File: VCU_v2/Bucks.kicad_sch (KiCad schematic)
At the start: 16 parts, among them U1 TPS5430

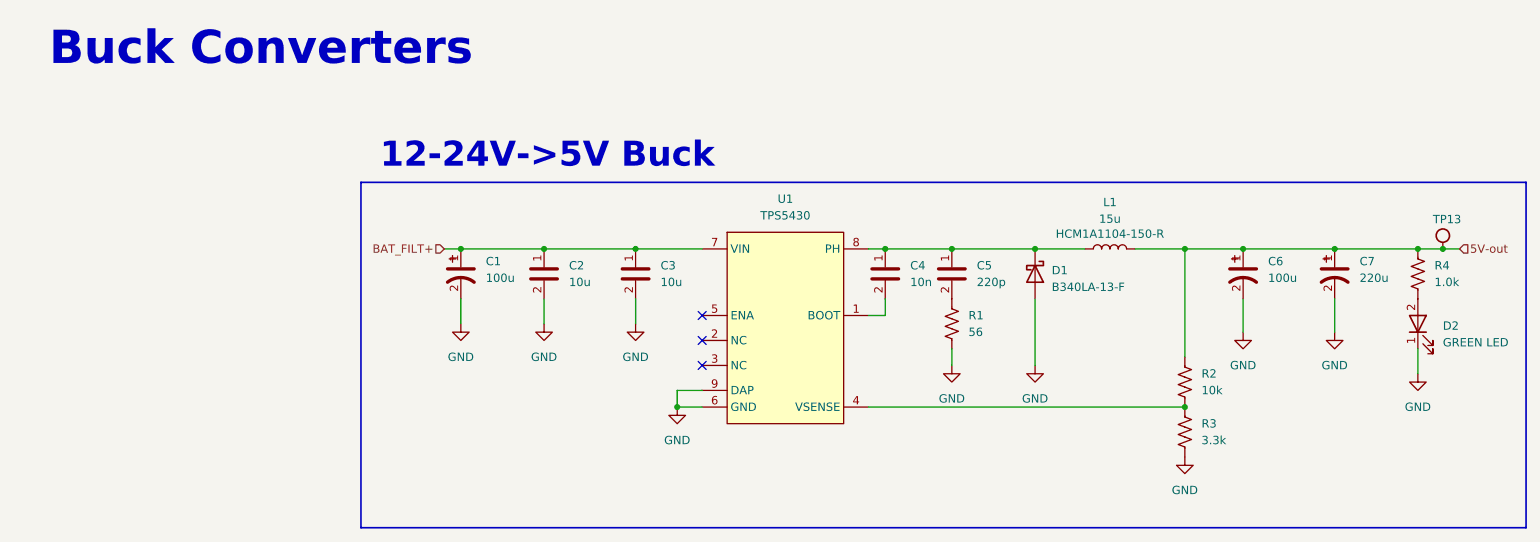
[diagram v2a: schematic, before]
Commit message: placements friggin 80% friggin done shoutout epstein
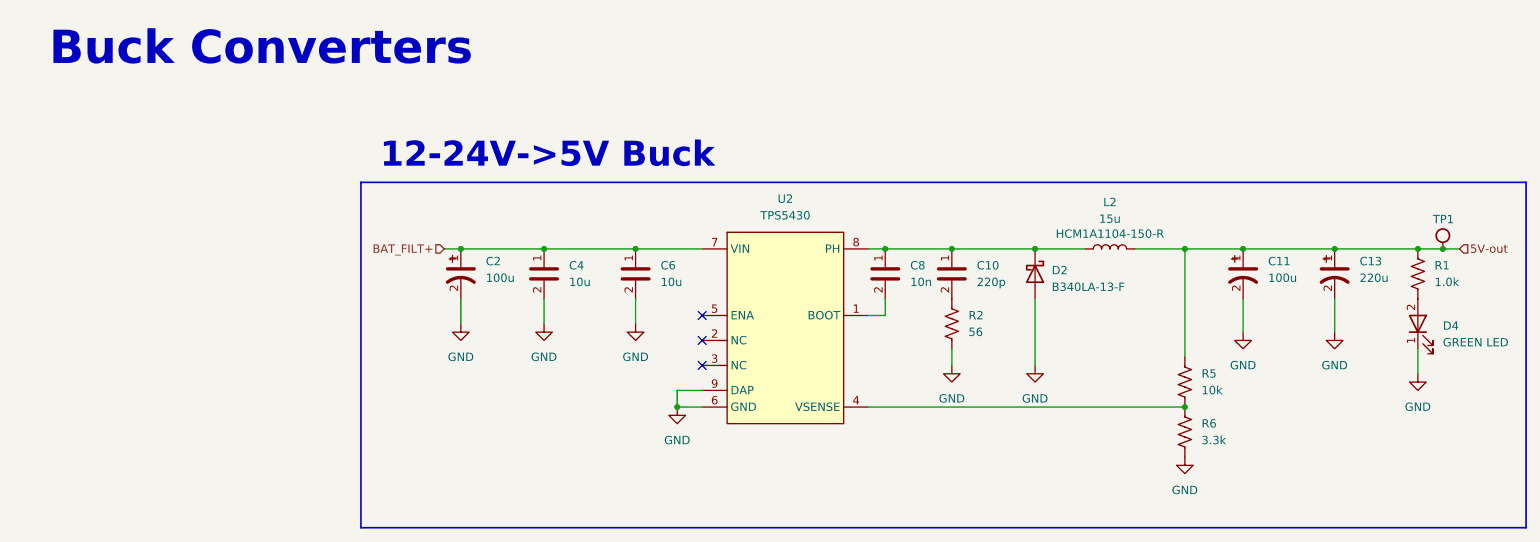
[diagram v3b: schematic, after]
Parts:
- renumbered C5 to C10, C6 to C11, C7 to C13, C1 to C2, C2 to C4, C3 to C6, C4 to C8, D1 to D2, D2 to D4, L1 to L2, R4 to R1, R1 to R2, R2 to R5, R3 to R6, TP13 to TP1, U1 to U2
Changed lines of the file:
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@@
 		(dnp no)
 		(fields_autoplaced yes)
-		(property "Reference" "#PWR017"
+		(property "Reference" "#PWR023"
 			(at 186.69 86.36 0)
 			(effects
@@
 			(project ""
 				(path "/4ee6c2ad-9a1b-4276-b3cf-1cc8dc52967e/9e4b5f8d-93dc-46d5-aa92-d0e0d2e07b3d/83ba1e49-760f-4968-9bbd-ff2e6c9ab433"
-					(reference "#PWR017")
+					(reference "#PWR023")
 					(unit 1)
 				)
@@
 		(dnp no)
 		(fields_autoplaced yes)
-		(property "Reference" "#PWR016"
+		(property "Reference" "#PWR021"
 			(at 163.83 72.39 0)
 			(effects
@@
 			(project "VCU_v1"
 				(path "/4ee6c2ad-9a1b-4276-b3cf-1cc8dc52967e/9e4b5f8d-93dc-46d5-aa92-d0e0d2e07b3d/83ba1e49-760f-4968-9bbd-ff2e6c9ab433"
-					(reference "#PWR016")
+					(reference "#PWR021")
 					(unit 1)
 				)
@@
 		(dnp no)
 		(fields_autoplaced yes)
-		(property "Reference" "#PWR012"
+		(property "Reference" "#PWR013"
 			(at 88.9 66.04 0)
 			(effects
@@
 			(project "VCU_v1"
 				(path "/4ee6c2ad-9a1b-4276-b3cf-1cc8dc52967e/9e4b5f8d-93dc-46d5-aa92-d0e0d2e07b3d/83ba1e49-760f-4968-9bbd-ff2e6c9ab433"
-					(reference "#PWR012")
+					(reference "#PWR013")
 					(unit 1)
 				)
@@
 		(dnp no)
 		(fields_autoplaced yes)
-		(property "Reference" "C3"
+		(property "Reference" "C6"
 			(at 106.68 50.7999 0)
 			(effects
@@
 			(project "VCU_v1"
 				(path "/4ee6c2ad-9a1b-4276-b3cf-1cc8dc52967e/9e4b5f8d-93dc-46d5-aa92-d0e0d2e07b3d/83ba1e49-760f-4968-9bbd-ff2e6c9ab433"
-					(reference "C3")
+					(reference "C6")
 					(unit 1)
 				)
@@
 		(on_board yes)
 		(dnp no)
-		(property "Reference" "D1"
+		(property "Reference" "D2"
 			(at 166.37 50.8 90)
 			(effects
@@
 			(project "VCU_v1"
 				(path "/4ee6c2ad-9a1b-4276-b3cf-1cc8dc52967e/9e4b5f8d-93dc-46d5-aa92-d0e0d2e07b3d/83ba1e49-760f-4968-9bbd-ff2e6c9ab433"
-					(reference "D1")
+					(reference "D2")
 					(unit 1)
 				)
@@
 		(dnp no)
 		(fields_autoplaced yes)
-		(property "Reference" "R1"
+		(property "Reference" "R2"
 			(at 153.67 58.4199 90)
 			(effects
@@
 			(project ""
 				(path "/4ee6c2ad-9a1b-4276-b3cf-1cc8dc52967e/9e4b5f8d-93dc-46d5-aa92-d0e0d2e07b3d/83ba1e49-760f-4968-9bbd-ff2e6c9ab433"
-					(reference "R1")
+					(reference "R2")
 					(unit 1)
 				)
@@
 		(dnp no)
 		(fields_autoplaced yes)
-		(property "Reference" "U1"
+		(property "Reference" "U2"
 			(at 125.73 40.64 0)
 			(effects
@@
 			(project "VCU_v1"
 				(path "/4ee6c2ad-9a1b-4276-b3cf-1cc8dc52967e/9e4b5f8d-93dc-46d5-aa92-d0e0d2e07b3d/83ba1e49-760f-4968-9bbd-ff2e6c9ab433"
-					(reference "U1")
+					(reference "U2")
 					(unit 1)
 				)
@@
 		(dnp no)
 		(fields_autoplaced yes)
-		(property "Reference" "C4"
+		(property "Reference" "C8"
 			(at 144.78 50.7999 0)
 			(effects
@@
 			(project "VCU_v1"
 				(path "/4ee6c2ad-9a1b-4276-b3cf-1cc8dc52967e/9e4b5f8d-93dc-46d5-aa92-d0e0d2e07b3d/83ba1e49-760f-4968-9bbd-ff2e6c9ab433"
-					(reference "C4")
+					(reference "C8")
 					(unit 1)
 				)
@@
 		(dnp no)
 		(fields_autoplaced yes)
-		(property "Reference" "#PWR014"
+		(property "Reference" "#PWR017"
 			(at 109.22 78.74 0)
 			(effects
@@
 			(project "VCU_v1"
 				(path "/4ee6c2ad-9a1b-4276-b3cf-1cc8dc52967e/9e4b5f8d-93dc-46d5-aa92-d0e0d2e07b3d/83ba1e49-760f-4968-9bbd-ff2e6c9ab433"
-					(reference "#PWR014")
+					(reference "#PWR017")
 					(unit 1)
 				)
@@
 		(dnp no)
 		(fields_autoplaced yes)
-		(property "Reference" "#PWR015"
+		(property "Reference" "#PWR019"
 			(at 151.13 72.39 0)
 			(effects
@@
 			(project "VCU_v1"
 				(path "/4ee6c2ad-9a1b-4276-b3cf-1cc8dc52967e/9e4b5f8d-93dc-46d5-aa92-d0e0d2e07b3d/83ba1e49-760f-4968-9bbd-ff2e6c9ab433"
-					(reference "#PWR015")
+					(reference "#PWR019")
 					(unit 1)
 				)
@@
 		(on_board yes)
 		(dnp no)
-		(property "Reference" "L1"
+		(property "Reference" "L2"
 			(at 175.26 41.148 90)
 			(effects
@@
 			(project ""
 				(path "/4ee6c2ad-9a1b-4276-b3cf-1cc8dc52967e/9e4b5f8d-93dc-46d5-aa92-d0e0d2e07b3d/83ba1e49-760f-4968-9bbd-ff2e6c9ab433"
-					(reference "L1")
+					(reference "L2")
 					(unit 1)
 				)
@@
 		(dnp no)
 		(fields_autoplaced yes)
-		(property "Reference" "R3"
+		(property "Reference" "R6"
 			(at 189.23 74.9299 90)
 			(effects
@@
 			(project ""
 				(path "/4ee6c2ad-9a1b-4276-b3cf-1cc8dc52967e/9e4b5f8d-93dc-46d5-aa92-d0e0d2e07b3d/83ba1e49-760f-4968-9bbd-ff2e6c9ab433"
-					(reference "R3")
+					(reference "R6")
 					(unit 1)
 				)
@@
 		(dnp no)
 		(fields_autoplaced yes)
-		(property "Reference" "C1"
+		(property "Reference" "C2"
 			(at 80.01 50.1649 0)
 			(effects
@@
 			(project ""
 				(path "/4ee6c2ad-9a1b-4276-b3cf-1cc8dc52967e/9e4b5f8d-93dc-46d5-aa92-d0e0d2e07b3d/83ba1e49-760f-4968-9bbd-ff2e6c9ab433"
-					(reference "C1")
+					(reference "C2")
 					(unit 1)
 				)
@@
 		(dnp no)
 		(fields_autoplaced yes)
-		(property "Reference" "R2"
+		(property "Reference" "R5"
 			(at 189.23 67.3099 90)
 			(effects
@@
 			(project ""
 				(path "/4ee6c2ad-9a1b-4276-b3cf-1cc8dc52967e/9e4b5f8d-93dc-46d5-aa92-d0e0d2e07b3d/83ba1e49-760f-4968-9bbd-ff2e6c9ab433"
-					(reference "R2")
+					(reference "R5")
 					(unit 1)
 				)
@@
 		(dnp no)
 		(fields_autoplaced yes)
-		(property "Reference" "C5"
+		(property "Reference" "C10"
 			(at 154.94 50.7999 0)
 			(effects
@@
 			(project ""
 				(path "/4ee6c2ad-9a1b-4276-b3cf-1cc8dc52967e/9e4b5f8d-93dc-46d5-aa92-d0e0d2e07b3d/83ba1e49-760f-4968-9bbd-ff2e6c9ab433"
-					(reference "C5")
+					(reference "C10")
 					(unit 1)
 				)
@@
 		(dnp no)
 		(fields_autoplaced yes)
-		(property "Reference" "#PWR019"
+		(property "Reference" "#PWR026"
 			(at 209.55 67.31 0)
 			(effects
@@
 			(project "VCU_v1"
 				(path "/4ee6c2ad-9a1b-4276-b3cf-1cc8dc52967e/9e4b5f8d-93dc-46d5-aa92-d0e0d2e07b3d/83ba1e49-760f-4968-9bbd-ff2e6c9ab433"
-					(reference "#PWR019")
+					(reference "#PWR026")
 					(unit 1)
 				)
@@
 		(dnp no)
 		(fields_autoplaced yes)
-		(property "Reference" "D2"
+		(property "Reference" "D4"
 			(at 226.06 60.0074 90)
 			(effects
@@
 			(project "VCU_v1"
 				(path "/4ee6c2ad-9a1b-4276-b3cf-1cc8dc52967e/9e4b5f8d-93dc-46d5-aa92-d0e0d2e07b3d/83ba1e49-760f-4968-9bbd-ff2e6c9ab433"
-					(reference "D2")
+					(reference "D4")
 					(unit 1)
 				)
@@
 		(on_board yes)
 		(dnp no)
-		(property "Reference" "TP13"
+		(property "Reference" "TP1"
 			(at 224.5368 43.0037 0)
 			(effects
@@
 			(project "VCU_v1"
 				(path "/4ee6c2ad-9a1b-4276-b3cf-1cc8dc52967e/9e4b5f8d-93dc-46d5-aa92-d0e0d2e07b3d/83ba1e49-760f-4968-9bbd-ff2e6c9ab433"
-					(reference "TP13")
+					(reference "TP1")
 					(unit 1)
 				)
@@
 		(dnp no)
 		(fields_autoplaced yes)
-		(property "Reference" "#PWR018"
+		(property "Reference" "#PWR024"
 			(at 195.58 67.31 0)
 			(effects
@@
 			(project "VCU_v1"
 				(path "/4ee6c2ad-9a1b-4276-b3cf-1cc8dc52967e/9e4b5f8d-93dc-46d5-aa92-d0e0d2e07b3d/83ba1e49-760f-4968-9bbd-ff2e6c9ab433"
-					(reference "#PWR018")
+					(reference "#PWR024")
 					(unit 1)
 				)
@@
 		(dnp no)
 		(fields_autoplaced yes)
-		(property "Reference" "C2"
+		(property "Reference" "C4"
 			(at 92.71 50.7999 0)
 			(effects
@@
 			(project "VCU_v1"
 				(path "/4ee6c2ad-9a1b-4276-b3cf-1cc8dc52967e/9e4b5f8d-93dc-46d5-aa92-d0e0d2e07b3d/83ba1e49-760f-4968-9bbd-ff2e6c9ab433"
-					(reference "C2")
+					(reference "C4")
 					(unit 1)
 				)
@@
 		(dnp no)
 		(fields_autoplaced yes)
-		(property "Reference" "#PWR020"
+		(property "Reference" "#PWR028"
 			(at 222.25 73.66 0)
 			(effects
@@
 			(project "VCU_v1"
 				(path "/4ee6c2ad-9a1b-4276-b3cf-1cc8dc52967e/9e4b5f8d-93dc-46d5-aa92-d0e0d2e07b3d/83ba1e49-760f-4968-9bbd-ff2e6c9ab433"
-					(reference "#PWR020")
+					(reference "#PWR028")
 					(unit 1)
 				)
@@
 		(dnp no)
 		(fields_autoplaced yes)
-		(property "Reference" "C7"
+		(property "Reference" "C13"
 			(at 213.36 50.1649 0)
 			(effects
@@
 			(project ""
 				(path "/4ee6c2ad-9a1b-4276-b3cf-1cc8dc52967e/9e4b5f8d-93dc-46d5-aa92-d0e0d2e07b3d/83ba1e49-760f-4968-9bbd-ff2e6c9ab433"
-					(reference "C7")
+					(reference "C13")
 					(unit 1)
 				)
@@
 		(dnp no)
 		(fields_autoplaced yes)
-		(property "Reference" "R4"
+		(property "Reference" "R1"
 			(at 224.79 50.7999 90)
 			(effects
@@
 			(project ""
 				(path "/4ee6c2ad-9a1b-4276-b3cf-1cc8dc52967e/9e4b5f8d-93dc-46d5-aa92-d0e0d2e07b3d/83ba1e49-760f-4968-9bbd-ff2e6c9ab433"
-					(reference "R4")
+					(reference "R1")
 					(unit 1)
 				)
@@
 		(dnp no)
 		(fields_autoplaced yes)
-		(property "Reference" "C6"
+		(property "Reference" "C11"
 			(at 199.39 50.1649 0)
 			(effects
@@
 			(project ""
 				(path "/4ee6c2ad-9a1b-4276-b3cf-1cc8dc52967e/9e4b5f8d-93dc-46d5-aa92-d0e0d2e07b3d/83ba1e49-760f-4968-9bbd-ff2e6c9ab433"
-					(reference "C6")
+					(reference "C11")
 					(unit 1)
 				)
@@
 		(dnp no)
 		(fields_autoplaced yes)
-		(property "Reference" "#PWR013"
+		(property "Reference" "#PWR015"
 			(at 102.87 66.04 0)
 			(effects
@@
 			(project "VCU_v1"
 				(path "/4ee6c2ad-9a1b-4276-b3cf-1cc8dc52967e/9e4b5f8d-93dc-46d5-aa92-d0e0d2e07b3d/83ba1e49-760f-4968-9bbd-ff2e6c9ab433"
-					(reference "#PWR013")
+					(reference "#PWR015")
 					(unit 1)
 				)
